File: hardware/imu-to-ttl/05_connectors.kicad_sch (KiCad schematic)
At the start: 10 parts, among them J3 J_NECK, J4 J_L, J5 J_R

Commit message: sync: 2026-10-12 日常更新
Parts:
- J3, J4, J5: footprint Connector_JST:JST_PH_B3B-PH-K_1x03_P2.00mm_Vertical -> Connector_PinHeader_2.54mm:PinHeader_1x03_P2.54mm_Horizontal
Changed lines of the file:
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@@
 	)
 	)
-		(property "Footprint" "Connector_JST:JST_PH_B3B-PH-K_1x03_P2.00mm_Vertical"
+		(property "Footprint" "Connector_PinHeader_2.54mm:PinHeader_1x03_P2.54mm_Horizontal"
 		(at 54.61 110.49 0)
 		(effects
@@
 	)
 	)
-		(property "Footprint" "Connector_JST:JST_PH_B3B-PH-K_1x03_P2.00mm_Vertical"
+		(property "Footprint" "Connector_PinHeader_2.54mm:PinHeader_1x03_P2.54mm_Horizontal"
 		(at 54.61 144.78 0)
 		(effects
@@
 	)
 	)
-		(property "Footprint" "Connector_JST:JST_PH_B3B-PH-K_1x03_P2.00mm_Vertical"
+		(property "Footprint" "Connector_PinHeader_2.54mm:PinHeader_1x03_P2.54mm_Horizontal"
 		(at 54.61 180.34 0)
 		(effects

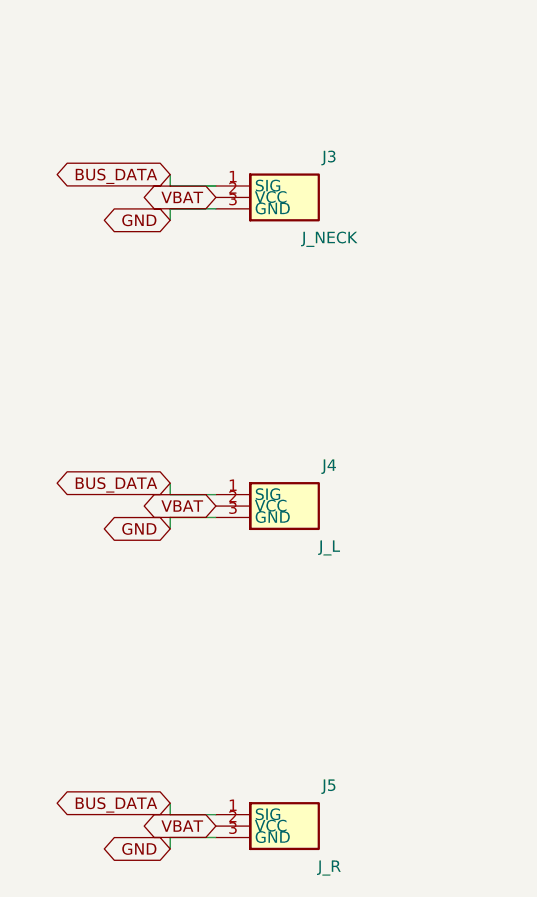
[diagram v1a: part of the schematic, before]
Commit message: sync: 2026-10-15 日常更新
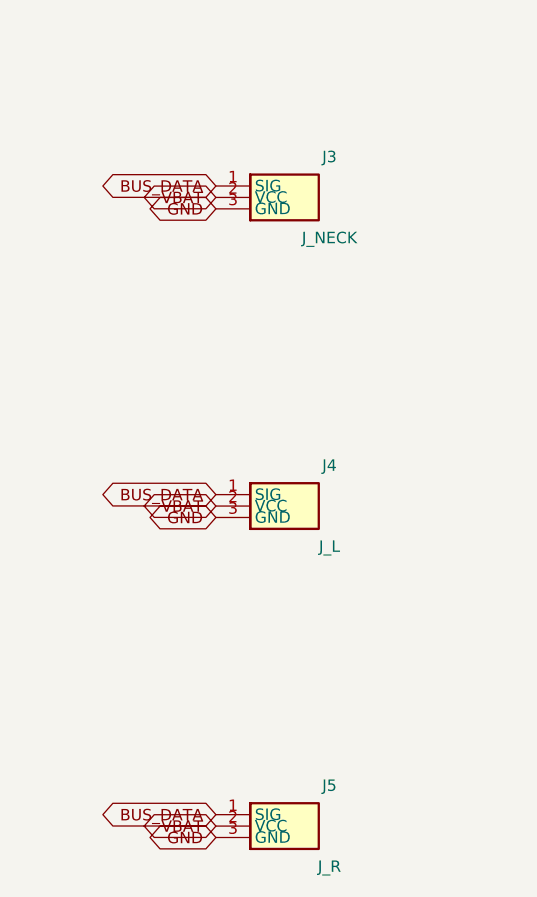
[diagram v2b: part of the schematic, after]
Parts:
- J3, J4, J5: footprint Connector_PinHeader_2.54mm:PinHeader_1x03_P2.54mm_Horizontal -> Connector_JST:JST_PH_B3B-PH-K_1x03_P2.00mm_Vertical
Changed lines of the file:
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@@
 	(global_label "BUS_DATA"
 		(shape bidirectional)
-		(at 41.91 107.95 180)
+		(at 46.99 109.22 180)
 		(fields_autoplaced yes)
 		(effects
@@
 	(global_label "GND"
 		(shape bidirectional)
-		(at 41.91 113.03 180)
+		(at 46.99 111.76 180)
 		(fields_autoplaced yes)
 		(effects
@@
 	(global_label "BUS_DATA"
 		(shape bidirectional)
-		(at 41.91 142.24 180)
+		(at 46.99 143.51 180)
 		(fields_autoplaced yes)
 		(effects
@@
 	(global_label "GND"
 		(shape bidirectional)
-		(at 41.91 147.32 180)
+		(at 46.99 146.05 180)
 		(fields_autoplaced yes)
 		(effects
@@
 	(global_label "BUS_DATA"
 		(shape bidirectional)
-		(at 41.91 177.80 180)
+		(at 46.99 179.07 180)
 		(fields_autoplaced yes)
 		(effects
@@
 	(global_label "GND"
 		(shape bidirectional)
-		(at 41.91 182.88 180)
+		(at 46.99 181.61 180)
 		(fields_autoplaced yes)
 		(effects
@@
 	)
 	)
-		(property "Footprint" "Connector_PinHeader_2.54mm:PinHeader_1x03_P2.54mm_Horizontal"
+		(property "Footprint" "Connector_JST:JST_PH_B3B-PH-K_1x03_P2.00mm_Vertical"
 		(at 54.61 110.49 0)
 		(effects
@@
 	)
 	)
-		(property "Footprint" "Connector_PinHeader_2.54mm:PinHeader_1x03_P2.54mm_Horizontal"
+		(property "Footprint" "Connector_JST:JST_PH_B3B-PH-K_1x03_P2.00mm_Vertical"
 		(at 54.61 144.78 0)
 		(effects
@@
 	)
 	)
-		(property "Footprint" "Connector_PinHeader_2.54mm:PinHeader_1x03_P2.54mm_Horizontal"
+		(property "Footprint" "Connector_JST:JST_PH_B3B-PH-K_1x03_P2.00mm_Vertical"
 		(at 54.61 180.34 0)
 		(effects
@@
 		)
 	)
-	(wire
-		(pts (xy 46.99 109.22) (xy 41.91 109.22))
-		(stroke
-			(width 0)
-			(type default)
-		)
-	)
-	(wire
-		(pts (xy 41.91 109.22) (xy 41.91 107.95))
-		(stroke
-			(width 0)
-			(type default)
-		)
-	)
-	(wire
-		(pts (xy 46.99 111.76) (xy 41.91 111.76))
-		(stroke
-			(width 0)
-			(type default)
-		)
-	)
-	(wire
-		(pts (xy 41.91 111.76) (xy 41.91 113.03))
-		(stroke
-			(width 0)
-			(type default)
-		)
-	)
-	(wire
-		(pts (xy 46.99 143.51) (xy 41.91 143.51))
-		(stroke
-			(width 0)
-			(type default)
-		)
-	)
-	(wire
-		(pts (xy 41.91 143.51) (xy 41.91 142.24))
-		(stroke
-			(width 0)
-			(type default)
-		)
-	)
-	(wire
-		(pts (xy 46.99 146.05) (xy 41.91 146.05))
-		(stroke
-			(width 0)
-			(type default)
-		)
-	)
-	(wire
-		(pts (xy 41.91 146.05) (xy 41.91 147.32))
-		(stroke
-			(width 0)
-			(type default)
-		)
-	)
-	(wire
-		(pts (xy 46.99 179.07) (xy 41.91 179.07))
-		(stroke
-			(width 0)
-			(type default)
-		)
-	)
-	(wire
-		(pts (xy 41.91 179.07) (xy 41.91 177.80))
-		(stroke
-			(width 0)
-			(type default)
-		)
-	)
-	(wire
-		(pts (xy 46.99 181.61) (xy 41.91 181.61))
-		(stroke
-			(width 0)
-			(type default)
-		)
-	)
-	(wire
-		(pts (xy 41.91 181.61) (xy 41.91 182.88))
-		(stroke
-			(width 0)
-			(type default)
-		)
-	)
-(embedded_fonts no)
+	(embedded_fonts no)
 )

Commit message: sync: 2026-10-15 日常更新
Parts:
- J3, J4, J5: footprint Connector_JST:JST_PH_B3B-PH-K_1x03_P2.00mm_Vertical -> imu_to_ttl:PinHeader_1x03_P2.54mm_Horizontal
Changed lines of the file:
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@@
 	)
 	)
-		(property "Footprint" "Connector_JST:JST_PH_B3B-PH-K_1x03_P2.00mm_Vertical"
+		(property "Footprint" "imu_to_ttl:PinHeader_1x03_P2.54mm_Horizontal"
 		(at 54.61 110.49 0)
 		(effects
@@
 	)
 	)
-		(property "Footprint" "Connector_JST:JST_PH_B3B-PH-K_1x03_P2.00mm_Vertical"
+		(property "Footprint" "imu_to_ttl:PinHeader_1x03_P2.54mm_Horizontal"
 		(at 54.61 144.78 0)
 		(effects
@@
 	)
 	)
-		(property "Footprint" "Connector_JST:JST_PH_B3B-PH-K_1x03_P2.00mm_Vertical"
+		(property "Footprint" "imu_to_ttl:PinHeader_1x03_P2.54mm_Horizontal"
 		(at 54.61 180.34 0)
 		(effects

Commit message: sync: 2026-10-15 日常更新
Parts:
- J3, J4, J5: LCSC C131339 -> C492411; MPN B3B-PH-K-S(LF)(SN) -> PZ254R-11-03P
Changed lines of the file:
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@@
 	)
 	)
-		(property "MPN" "B3B-PH-K-S(LF)(SN)"
+		(property "MPN" "PZ254R-11-03P"
 		(at 54.61 110.49 0)
 		(effects
@@
 	)
 	)
-		(property "LCSC" "C131339"
+		(property "LCSC" "C492411"
 		(at 54.61 110.49 0)
 		(effects
@@
 	)
 	)
-		(property "MPN" "B3B-PH-K-S(LF)(SN)"
+		(property "MPN" "PZ254R-11-03P"
 		(at 54.61 144.78 0)
 		(effects
@@
 	)
 	)
-		(property "LCSC" "C131339"
+		(property "LCSC" "C492411"
 		(at 54.61 144.78 0)
 		(effects
@@
 	)
 	)
-		(property "MPN" "B3B-PH-K-S(LF)(SN)"
+		(property "MPN" "PZ254R-11-03P"
 		(at 54.61 180.34 0)
 		(effects
@@
 	)
 	)
-		(property "LCSC" "C131339"
+		(property "LCSC" "C492411"
 		(at 54.61 180.34 0)
 		(effects

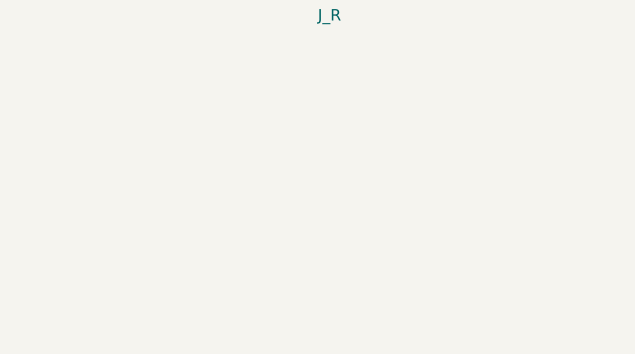
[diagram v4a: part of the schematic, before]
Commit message: sync: 2026-10-21 日常更新
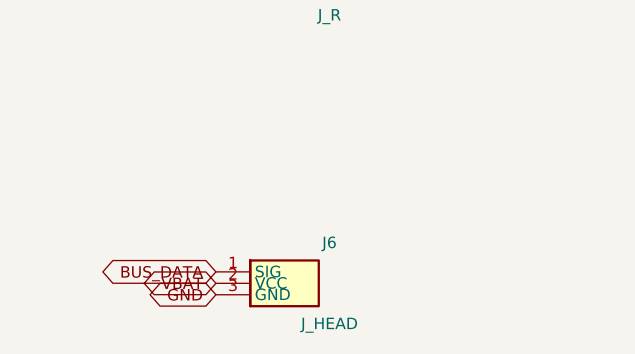
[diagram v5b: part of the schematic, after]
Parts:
- added J6: J_HEAD, imu_to_ttl:CONN-TH_B3B-PH-K-S, symbol imu_ttl:JST_PH_B3B_3P
- J3, J4, J5: footprint imu_to_ttl:PinHeader_1x03_P2.54mm_Horizontal -> imu_to_ttl:CONN-TH_B3B-PH-K-S; LCSC C492411 -> C131339; MPN PZ254R-11-03P -> B3B-PH-K-S(LF)(SN)
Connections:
- net BUS_DATA: now also J6.1 (SIG)
- net GND: now also J6.3 (GND)
- net VBAT: now also J6.2 (VCC)
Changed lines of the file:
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@@
+	)
+	)
+	(global_label "BUS_DATA"
+		(shape bidirectional)
+		(at 46.99 213.36 180)
+		(fields_autoplaced yes)
+		(effects
+		(font
+			(size 1.27 1.27)
+		)
+			(justify right)
+	)
+	)
+	(global_label "VBAT"
+		(shape bidirectional)
+		(at 46.99 214.63 180)
+		(fields_autoplaced yes)
+		(effects
+		(font
+			(size 1.27 1.27)
+		)
+			(justify right)
+	)
+	)
+	(global_label "GND"
+		(shape bidirectional)
+		(at 46.99 215.9 180)
+		(fields_autoplaced yes)
+		(effects
+		(font
+			(size 1.27 1.27)
+		)
+			(justify right)
 	)
 	)
@@
 	)
 	)
-		(property "Footprint" "imu_to_ttl:PinHeader_1x03_P2.54mm_Horizontal"
+		(property "Footprint" "imu_to_ttl:CONN-TH_B3B-PH-K-S"
 		(at 54.61 110.49 0)
 		(effects
@@
 	)
 	)
-		(property "MPN" "PZ254R-11-03P"
-		(at 54.61 110.49 0)
-		(effects
-		(font
-			(size 1.27 1.27)
-		)
-			(hide yes)
-	)
-	)
-		(property "LCSC" "C492411"
+		(property "MPN" "B3B-PH-K-S(LF)(SN)"
+		(at 54.61 110.49 0)
+		(effects
+		(font
+			(size 1.27 1.27)
+		)
+			(hide yes)
+	)
+	)
+		(property "LCSC" "C131339"
 		(at 54.61 110.49 0)
 		(effects
@@
 	)
 	)
-		(property "Footprint" "imu_to_ttl:PinHeader_1x03_P2.54mm_Horizontal"
+		(property "Footprint" "imu_to_ttl:CONN-TH_B3B-PH-K-S"
 		(at 54.61 144.78 0)
 		(effects
@@
 	)
 	)
-		(property "MPN" "PZ254R-11-03P"
-		(at 54.61 144.78 0)
-		(effects
-		(font
-			(size 1.27 1.27)
-		)
-			(hide yes)
-	)
-	)
-		(property "LCSC" "C492411"
+		(property "MPN" "B3B-PH-K-S(LF)(SN)"
+		(at 54.61 144.78 0)
+		(effects
+		(font
+			(size 1.27 1.27)
+		)
+			(hide yes)
+	)
+	)
+		(property "LCSC" "C131339"
 		(at 54.61 144.78 0)
 		(effects
@@
 	)
 	)
-		(property "Footprint" "imu_to_ttl:PinHeader_1x03_P2.54mm_Horizontal"
+		(property "Footprint" "imu_to_ttl:CONN-TH_B3B-PH-K-S"
 		(at 54.61 180.34 0)
 		(effects
@@
 	)
 	)
-		(property "MPN" "PZ254R-11-03P"
-		(at 54.61 180.34 0)
-		(effects
-		(font
-			(size 1.27 1.27)
-		)
-			(hide yes)
-	)
-	)
-		(property "LCSC" "C492411"
+		(property "MPN" "B3B-PH-K-S(LF)(SN)"
+		(at 54.61 180.34 0)
+		(effects
+		(font
+			(size 1.27 1.27)
+		)
+			(hide yes)
+	)
+	)
+		(property "LCSC" "C131339"
 		(at 54.61 180.34 0)
 		(effects
@@
 					(unit 1)
 				)
+			)
+		)
+	)
+	(symbol
+		(lib_id "imu_ttl:JST_PH_B3B_3P")
+		(at 54.61 214.63 0)
+		(unit 1)
+		(exclude_from_sim no)
+		(in_bom yes)
+		(on_board yes)
+		(dnp no)
+		(property "Reference" "J6"
+		(at 59.61 210.13 0)
+		(effects
+		(font
+			(size 1.27 1.27)
+		)
+	)
+	)
+		(property "Value" "J_HEAD"
+		(at 59.61 219.13 0)
+		(effects
+		(font
+			(size 1.27 1.27)
+		)
+	)
+	)
+		(property "Footprint" "imu_to_ttl:CONN-TH_B3B-PH-K-S"
+		(at 54.61 214.63 0)
+		(effects
+		(font
+			(size 1.27 1.27)
+		)
+			(hide yes)
+	)
+	)
+		(property "Datasheet" "~"
+		(at 54.61 214.63 0)
+		(effects
+		(font
+			(size 1.27 1.27)
+		)
+			(hide yes)
+	)
+	)
+		(property "Description" "v3.7 head/spare branch"
+		(at 54.61 214.63 0)
+		(effects
+		(font
+			(size 1.27 1.27)
+		)
+			(hide yes)
+	)
+	)
+		(property "MPN" "B3B-PH-K-S(LF)(SN)"
+		(at 54.61 214.63 0)
+		(effects
+		(font
+			(size 1.27 1.27)
+		)
+			(hide yes)
+	)
+	)
+		(property "LCSC" "C131339"
+		(at 54.61 214.63 0)
+		(effects
+		(font
+			(size 1.27 1.27)
+		)
+			(hide yes)
+	)
+	)
+		(pin "1"
+		)
+		(pin "2"
+		)
+		(pin "3"
+		)
+		(instances
+			(project "imu_to_ttl"
+				(path "/3d3ee743-797d-5481-a518-f87a3584d0e2/d10532dc-e93c-5500-9b16-6fc2a6d8f858/cbcc4736-458d-5853-bb3f-0254cf353dd8"
+					(reference "J6")
+					(unit 1)
+				)

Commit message: sync: 2026-10-30 日常更新
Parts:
- J4, J5: footprint imu_to_ttl:CONN-TH_B3B-PH-K-S -> imu_to_ttl:CONN-TH_S3B-PH-K-S; LCSC C131339 -> C169277; MPN B3B-PH-K-S(LF)(SN) -> S3B-PH-K-S(LF)(SN)
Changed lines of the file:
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@@
 	)
 	)
-		(property "Footprint" "imu_to_ttl:CONN-TH_B3B-PH-K-S"
+		(property "Footprint" "imu_to_ttl:CONN-TH_S3B-PH-K-S"
 		(at 54.61 144.78 0)
 		(effects
@@
 	)
 	)
-		(property "Description" "left leg 20-24"
+		(property "Description" "left leg 20-24 (v3.8 side entry)"
 		(at 54.61 144.78 0)
 		(effects
@@
 	)
 	)
-		(property "MPN" "B3B-PH-K-S(LF)(SN)"
+		(property "MPN" "S3B-PH-K-S(LF)(SN)"
 		(at 54.61 144.78 0)
 		(effects
@@
 	)
 	)
-		(property "LCSC" "C131339"
+		(property "LCSC" "C169277"
 		(at 54.61 144.78 0)
 		(effects
@@
 	)
 	)
-		(property "Footprint" "imu_to_ttl:CONN-TH_B3B-PH-K-S"
+		(property "Footprint" "imu_to_ttl:CONN-TH_S3B-PH-K-S"
 		(at 54.61 180.34 0)
 		(effects
@@
 	)
 	)
-		(property "Description" "right leg 10-14"
+		(property "Description" "right leg 10-14 (v3.8 side entry)"
 		(at 54.61 180.34 0)
 		(effects
@@
 	)
 	)
-		(property "MPN" "B3B-PH-K-S(LF)(SN)"
+		(property "MPN" "S3B-PH-K-S(LF)(SN)"
 		(at 54.61 180.34 0)
 		(effects
@@
 	)
 	)
-		(property "LCSC" "C131339"
+		(property "LCSC" "C169277"
 		(at 54.61 180.34 0)
 		(effects
